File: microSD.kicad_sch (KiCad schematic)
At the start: 3 parts, among them J16 Micro_SD_Card_Det

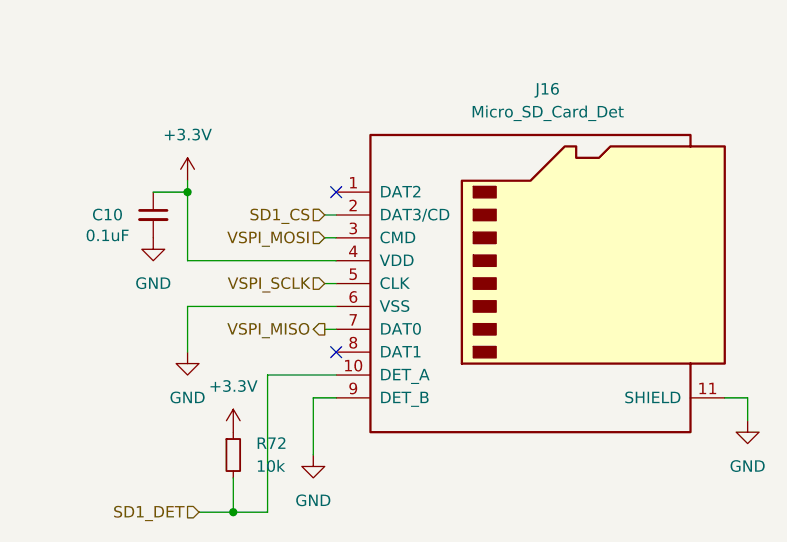
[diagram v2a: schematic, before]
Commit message: commit
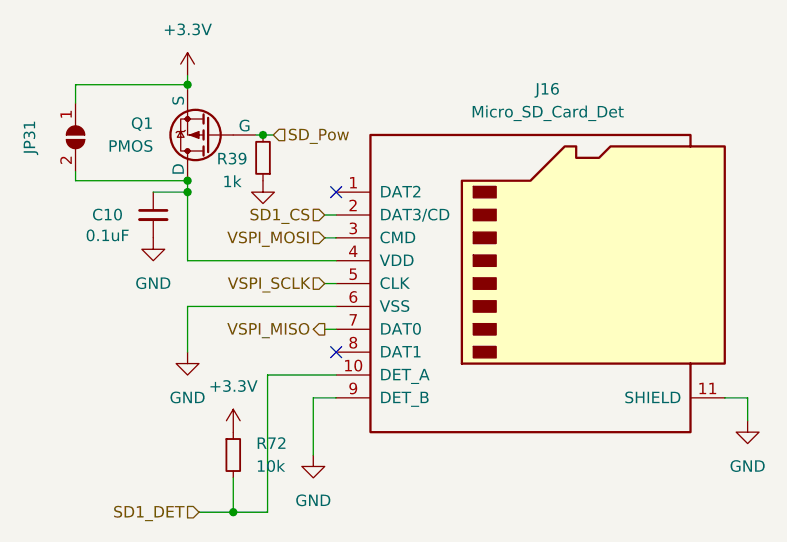
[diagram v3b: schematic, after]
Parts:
- added JP31: SolderJumper_2_Open, iclr:SmallerSolderJP, symbol Jumper:SolderJumper_2_Open
- added Q1: PMOS, Package_TO_SOT_SMD:SOT-723, symbol Simulation_SPICE:PMOS
- added R39: 1k, Resistor_SMD:R_0402_1005Metric, symbol Device:R_Small
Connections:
- net +3V3: now also JP31.1 (A), Q1.3 (S); no longer C10.1, J16.4 (VDD)
- net GND: now also R39.1
- new net: C10.1, J16.4 (VDD), JP31.2 (B), Q1.1 (D)
- new net SD_Pow: Q1.2 (G), R39.2
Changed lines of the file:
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@@
 (kicad_sch (version 20230121) (generator eeschema)
   (paper "A4")
+  (junction (at 108.204 59.69) (diameter 0) (color 0 0 0 0)
+  )
+  (junction (at 99.822 54.102) (diameter 0) (color 0 0 0 0)
+  )
   (junction (at 104.902 101.6) (diameter 0) (color 0 0 0 0)
   )
   (junction (at 99.822 66.04) (diameter 0) (color 0 0 0 0)
+  )
+  (junction (at 99.822 64.77) (diameter 0) (color 0 0 0 0)
   )
   (no_connect (at 116.332 83.82))
   (no_connect (at 116.332 66.04))
+  (wire (pts (xy 99.822 64.77) (xy 87.376 64.77))
+    (stroke (width 0) (type default))
+  )
+  (wire (pts (xy 87.376 54.102) (xy 99.822 54.102))
+    (stroke (width 0) (type default))
+  )
   (wire (pts (xy 115.062 68.58) (xy 116.332 68.58))
     (stroke (width 0) (type default))
@@
     (stroke (width 0) (type default))
   )
+  (wire (pts (xy 87.376 56.134) (xy 87.376 54.102))
+    (stroke (width 0) (type default))
+  )
   (wire (pts (xy 99.822 66.04) (xy 99.822 73.66))
     (stroke (width 0) (type default))
@@
     (stroke (width 0) (type default))
   )
+  (wire (pts (xy 99.822 53.086) (xy 99.822 54.102))
+    (stroke (width 0) (type default))
+  )
   (wire (pts (xy 101.092 101.6) (xy 104.902 101.6))
     (stroke (width 0) (type default))
@@
     (stroke (width 0) (type default))
   )
+  (wire (pts (xy 107.442 59.69) (xy 108.204 59.69))
+    (stroke (width 0) (type default))
+  )
   (wire (pts (xy 108.712 86.36) (xy 108.712 101.6))
     (stroke (width 0) (type default))
@@
     (stroke (width 0) (type default))
   )
+  (wire (pts (xy 108.204 59.69) (xy 109.347 59.69))
+    (stroke (width 0) (type default))
+  )
+  (wire (pts (xy 87.376 64.77) (xy 87.376 63.754))
+    (stroke (width 0) (type default))
+  )
+  (wire (pts (xy 99.822 54.102) (xy 99.822 54.61))
+    (stroke (width 0) (type default))
+  )
   (wire (pts (xy 159.512 88.9) (xy 162.052 88.9))
     (stroke (width 0) (type default))
+  )
+  (hierarchical_label "SD_Pow" (shape input) (at 109.347 59.69 0) (fields_autoplaced)
+    (effects (font (size 1.27 1.27)) (justify left))
   )
   (hierarchical_label "VSPI_SCLK" (shape input) (at 115.062 76.2 180) (fields_autoplaced)
@@
     )
   )
+  (symbol (lib_id "power:GND") (at 108.204 64.77 0) (unit 1)
+    (in_bom yes) (on_board yes) (dnp no) (fields_autoplaced)
+    (property "Reference" "#PWR085" (at 108.204 71.12 0)
+      (effects (font (size 1.27 1.27)) hide)
+    )
+    (property "Value" "GND" (at 110.109 66.4738 0)
+      (effects (font (size 1.27 1.27)) (justify left) hide)
+    )
+    (property "Footprint" "" (at 108.204 64.77 0)
+      (effects (font (size 1.27 1.27)) hide)
+    )
+    (property "Datasheet" "" (at 108.204 64.77 0)
+      (effects (font (size 1.27 1.27)) hide)
+    )
+    (pin "1")
+    (instances
+      (project "Ricardo-Stark"
+        (path "/7db990e4-92e1-4f99-b4d2-435bbec1ba83/cbb4aecb-b4d4-4eab-8e16-74accf8129be"
+          (reference "#PWR030") (unit 1)
+        )
+      )
+    )
+  )
   (symbol (lib_id "power:+3.3V") (at 104.902 92.71 0) (unit 1)
     (in_bom yes) (on_board yes) (dnp no) (fields_autoplaced)
@@
     )
   )
-  (symbol (lib_id "power:+3.3V") (at 99.822 64.77 0) (unit 1)
-    (in_bom yes) (on_board yes) (dnp no) (fields_autoplaced)
-    (property "Reference" "#PWR0157" (at 99.822 68.58 0)
-      (effects (font (size 1.27 1.27)) hide)
-    )
-    (property "Value" "+3.3V" (at 99.822 59.69 0)
-      (effects (font (size 1.27 1.27)))
-    )
-    (property "Footprint" "" (at 99.822 64.77 0)
-      (effects (font (size 1.27 1.27)) hide)
-    )
-    (property "Datasheet" "" (at 99.822 64.77 0)
-      (effects (font (size 1.27 1.27)) hide)
-    )
-    (pin "1")
-    (instances
-      (project "sensorboard"
-        (path "/26801cfb-b53b-4a6a-a2f4-5f4986565765/f50ea3f6-9887-4dc3-9ec9-7a0fb1ee7721"
-          (reference "#PWR0157") (unit 1)
-        )
-      )
-      (project "Ricardo-Stark"
-        (path "/7db990e4-92e1-4f99-b4d2-435bbec1ba83/cbb4aecb-b4d4-4eab-8e16-74accf8129be"
-          (reference "#PWR0169") (unit 1)
+  (symbol (lib_id "Jumper:SolderJumper_2_Open") (at 87.376 59.944 270) (unit 1)
+    (in_bom yes) (on_board yes) (dnp no)
+    (property "Reference" "JP31" (at 82.296 59.944 0)
+      (effects (font (size 1.27 1.27)))
+    )
+    (property "Value" "SolderJumper_2_Open" (at 55.626 42.164 0)
+      (effects (font (size 1.27 1.27)) hide)
+    )
+    (property "Footprint" "iclr:SmallerSolderJP" (at 87.376 59.944 0)
+      (effects (font (size 1.27 1.27)) hide)
+    )
+    (property "Datasheet" "~" (at 87.376 59.944 0)
+      (effects (font (size 1.27 1.27)) hide)
+    )
+    (pin "1")
+    (pin "2")
+    (instances
+      (project "sensorboard - Copy"
+        (path "/26801cfb-b53b-4a6a-a2f4-5f4986565765/00000000-0000-0000-0000-000061b9f0c0"
+          (reference "JP31") (unit 1)
+        )
+      )
+      (project "Ricardo-Stark"
+        (path "/7db990e4-92e1-4f99-b4d2-435bbec1ba83/249a9f46-b59f-4de1-97d1-386ac76339a5"
+          (reference "JP27") (unit 1)
+        )
+        (path "/7db990e4-92e1-4f99-b4d2-435bbec1ba83/cbb4aecb-b4d4-4eab-8e16-74accf8129be"
+          (reference "JP3") (unit 1)
         )
       )
@@
         )
       )
+    )
+  )
+  (symbol (lib_id "power:+3.3V") (at 99.822 53.086 0) (unit 1)
+    (in_bom yes) (on_board yes) (dnp no) (fields_autoplaced)
+    (property "Reference" "#PWR0159" (at 99.822 56.896 0)
+      (effects (font (size 1.27 1.27)) hide)
+    )
+    (property "Value" "+3.3V" (at 99.822 48.006 0)
+      (effects (font (size 1.27 1.27)))
+    )
+    (property "Footprint" "" (at 99.822 53.086 0)
+      (effects (font (size 1.27 1.27)) hide)
+    )
+    (property "Datasheet" "" (at 99.822 53.086 0)
+      (effects (font (size 1.27 1.27)) hide)
+    )
+    (pin "1")
+    (instances
+      (project "sensorboard"
+        (path "/26801cfb-b53b-4a6a-a2f4-5f4986565765/f50ea3f6-9887-4dc3-9ec9-7a0fb1ee7721"
+          (reference "#PWR0159") (unit 1)
+        )
+      )
+      (project "Ricardo-Stark"
+        (path "/7db990e4-92e1-4f99-b4d2-435bbec1ba83/cbb4aecb-b4d4-4eab-8e16-74accf8129be"
+          (reference "#PWR031") (unit 1)
+        )
+      )
+    )
+  )
+  (symbol (lib_id "Device:R_Small") (at 108.204 62.23 180) (unit 1)
+    (in_bom yes) (on_board yes) (dnp no)
+    (property "Reference" "R39" (at 104.775 62.3601 0)
+      (effects (font (size 1.27 1.27)))
+    )
+    (property "Value" "1k" (at 104.775 64.897 0)
+      (effects (font (size 1.27 1.27)))
+    )
+    (property "Footprint" "Resistor_SMD:R_0402_1005Metric" (at 108.204 62.23 0)
+      (effects (font (size 1.27 1.27)) hide)
+    )
+    (property "Datasheet" "~" (at 108.204 62.23 0)
+      (effects (font (size 1.27 1.27)) hide)
+    )
+    (pin "1")
+    (pin "2")
+    (instances
+      (project "Ricardo-Stark"
+        (path "/7db990e4-92e1-4f99-b4d2-435bbec1ba83/cbb4aecb-b4d4-4eab-8e16-74accf8129be"
+          (reference "R14") (unit 1)
+        )
+      )
+    )
+  )
+  (symbol (lib_id "Simulation_SPICE:PMOS") (at 102.362 59.69 180) (unit 1)
+    (in_bom yes) (on_board yes) (dnp no) (fields_autoplaced)
+    (property "Reference" "Q1" (at 96.012 58.42 0)
+      (effects (font (size 1.27 1.27)) (justify left))
+    )
+    (property "Value" "PMOS" (at 96.012 60.96 0)
+      (effects (font (size 1.27 1.27)) (justify left))
+    )
+    (property "Footprint" "Package_TO_SOT_SMD:SOT-723" (at 97.282 62.23 0)
+      (effects (font (size 1.27 1.27)) hide)
+    )
+    (property "Datasheet" "https://ngspice.sourceforge.io/docs/ngspice-manual.pdf" (at 102.362 46.99 0)
+      (effects (font (size 1.27 1.27)) hide)
+    )
+    (property "Sim.Device" "PMOS" (at 102.362 42.545 0)
+      (effects (font (size 1.27 1.27)) hide)
+    )
+    (property "Sim.Type" "VDMOS" (at 102.362 40.64 0)
+      (effects (font (size 1.27 1.27)) hide)
+    )
+    (property "Sim.Pins" "1=D 2=G 3=S" (at 102.362 44.45 0)
+      (effects (font (size 1.27 1.27)) hide)
+    )
+    (pin "2")
+    (pin "3")
+    (pin "1")
+    (instances
+      (project "Ricardo-Stark"
+        (path "/7db990e4-92e1-4f99-b4d2-435bbec1ba83/cbb4aecb-b4d4-4eab-8e16-74accf8129be"
+          (reference "Q1") (unit 1)
+        )
+      )
